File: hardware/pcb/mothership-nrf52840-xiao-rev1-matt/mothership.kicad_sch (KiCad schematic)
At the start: 46 parts, among them J1 HRO TYPE-C-31-M-12, J10 Screw_Terminal_ADB_SHIELD, J11 Screw_Terminal_ADB_VCC, J12 USB_FLEX_ADAPTER_SOLDER_PADS_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, J2 USB_FLEX_ADAPTER_SOLDER_PADS, J3 CONN_BATT, J4 CONN_MATRIX_BOT_L, J5 CONN_MATRIX_BOT_R, J6 CONN_MATRIX_TOP_L, J7 CONN_MATRIX_TOP_R, J8 SPI, J9 EC11, Q1 AO3401A, Q2 FDC6305N, SW1 SW_PWR, SW2 SW_EXT_RST, U1 NCP361SN, U2 XIAO_nRF52840, U3 MCP23017x-x-SS, U4 MCP23017x-x-SS, U5 DT1452-02SO, U6 HY2115-LB9D

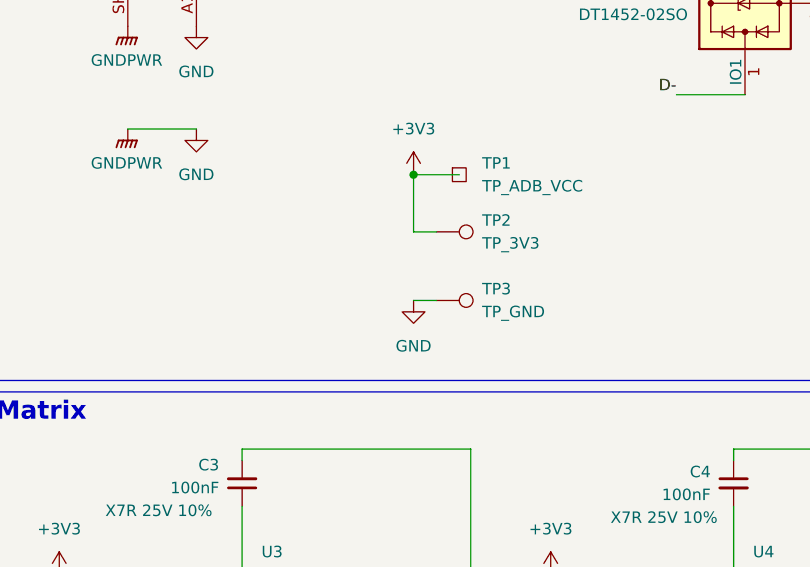
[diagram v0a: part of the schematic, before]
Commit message: sch: finalize the sch
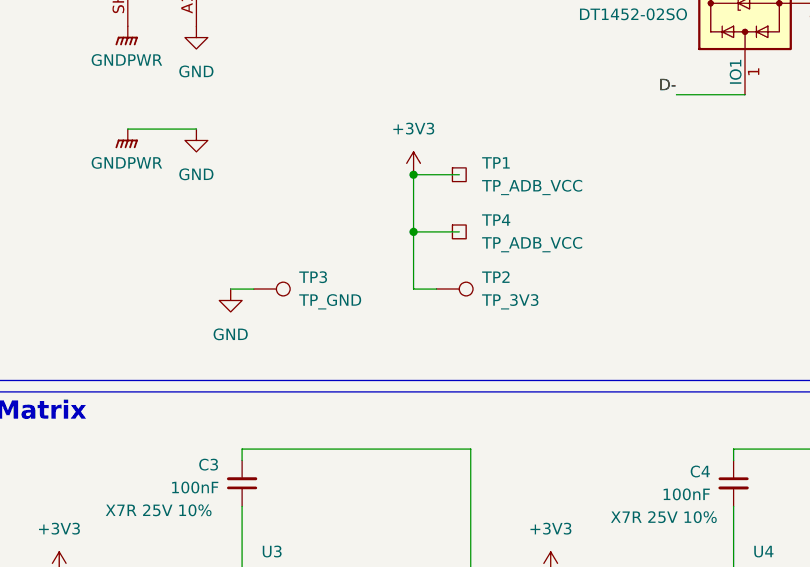
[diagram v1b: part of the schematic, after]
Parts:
- added TP4: TP_ADB_VCC, A9M0330:TestPoint_Pad_2.5x2.5mm, symbol A9M0330:TestPoint_Square
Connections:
- net +3V3: now also TP4.1
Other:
- moved on the sheet: TP3
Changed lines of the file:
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@@
 	)
 	(junction
+		(at 59.69 88.9)
+		(diameter 0)
+		(color 0 0 0 0)
+	)
+	(junction
 		(at 132.08 27.94)
 		(diameter 0)
@@
 	(wire
 		(pts
+			(xy 59.69 88.9) (xy 59.69 95.25)
+		)
+		(stroke
+			(width 0)
+			(type default)
+		)
+	)
+	(wire
+		(pts
 			(xy 140.97 60.96) (xy 140.97 62.23)
 		)
@@
 	(wire
 		(pts
+			(xy 59.69 95.25) (xy 62.23 95.25)
+		)
+		(stroke
+			(width 0)
+			(type default)
+		)
+	)
+	(wire
+		(pts
 			(xy 59.69 236.22) (xy 59.69 240.03)
 		)
@@
 	(wire
 		(pts
-			(xy 59.69 96.52) (xy 62.23 96.52)
+			(xy 39.37 95.25) (xy 41.91 95.25)
 		)
 		(stroke
@@
 	(wire
 		(pts
-			(xy 59.69 88.9) (xy 62.23 88.9)
+			(xy 59.69 88.9) (xy 64.77 88.9)
 		)
 		(stroke
@@
 	)
 	(symbol
+		(lib_id "A9M0330:TestPoint")
+		(at 62.23 95.25 270)
+		(unit 1)
+		(body_style 1)
+		(exclude_from_sim no)
+		(in_bom yes)
+		(on_board yes)
+		(in_pos_files yes)
+		(dnp no)
+		(fields_autoplaced yes)
+		(property "Reference" "TP2"
+			(at 67.31 93.9799 90)
+			(show_name no)
+			(do_not_autoplace no)
+			(effects
+				(font
+					(size 1.27 1.27)
+				)
+				(justify left)
+			)
+		)
+		(property "Value" "TP_3V3"
+			(at 67.31 96.5199 90)
+			(show_name no)
+			(do_not_autoplace no)
+			(effects
+				(font
+					(size 1.27 1.27)
+				)
+				(justify left)
+			)
+		)
+		(property "Footprint" "A9M0330:TestPoint_THTPad_D2.0mm_Drill1.0mm"
+			(at 62.23 100.33 0)
+			(hide yes)
+			(show_name no)
+			(do_not_autoplace no)
+			(effects
+				(font
+					(size 1.27 1.27)
+				)
+			)
+		)
+		(property "Datasheet" ""
+			(at 62.23 100.33 0)
+			(hide yes)
+			(show_name no)
+			(do_not_autoplace no)
+			(effects
+				(font
+					(size 1.27 1.27)
+				)
+			)
+		)
+		(property "Description" "test point"
+			(at 62.23 95.25 0)
+			(hide yes)
+			(show_name no)
+			(do_not_autoplace no)
+			(effects
+				(font
+					(size 1.27 1.27)
+				)
+			)
+		)
+		(pin "1"
+		)
+		(instances
+			(project "mothership"
+				(path "/02dc08fe-8ec4-4078-b85a-ecd1690e4fdc"
+					(reference "TP2")
+					(unit 1)
+				)
+			)
+		)
+	)
+	(symbol
 		(lib_id "power:+3V3")
 		(at 74.93 127 0)
@@
 	)
 	(symbol
-		(lib_id "A9M0330:TestPoint")
-		(at 62.23 88.9 270)
-		(unit 1)
-		(body_style 1)
-		(exclude_from_sim no)
-		(in_bom yes)
-		(on_board yes)
-		(in_pos_files yes)
-		(dnp no)
-		(fields_autoplaced yes)
-		(property "Reference" "TP2"
-			(at 67.31 87.6299 90)
-			(show_name no)
-			(do_not_autoplace no)
-			(effects
-				(font
-					(size 1.27 1.27)
-				)
-				(justify left)
-			)
-		)
-		(property "Value" "TP_3V3"
-			(at 67.31 90.1699 90)
-			(show_name no)
-			(do_not_autoplace no)
-			(effects
-				(font
-					(size 1.27 1.27)
-				)
-				(justify left)
-			)
-		)
-		(property "Footprint" "A9M0330:TestPoint_THTPad_D2.0mm_Drill1.0mm"
-			(at 62.23 93.98 0)
-			(hide yes)
-			(show_name no)
-			(do_not_autoplace no)
-			(effects
-				(font
-					(size 1.27 1.27)
-				)
-			)
-		)
-		(property "Datasheet" ""
-			(at 62.23 93.98 0)
-			(hide yes)
-			(show_name no)
-			(do_not_autoplace no)
-			(effects
-				(font
-					(size 1.27 1.27)
-				)
-			)
-		)
-		(property "Description" "test point"
-			(at 62.23 88.9 0)
-			(hide yes)
-			(show_name no)
-			(do_not_autoplace no)
-			(effects
-				(font
-					(size 1.27 1.27)
-				)
-			)
-		)
-		(pin "1"
-		)
-		(instances
-			(project "mothership"
-				(path "/02dc08fe-8ec4-4078-b85a-ecd1690e4fdc"
-					(reference "TP2")
-					(unit 1)
-				)
-			)
-		)
-	)
-	(symbol
 		(lib_id "power:GND")
 		(at 337.82 147.32 0)
@@
 	(symbol
 		(lib_id "power:GND")
-		(at 59.69 96.52 0)
+		(at 39.37 95.25 0)
 		(unit 1)
 		(body_style 1)
@@
 		(fields_autoplaced yes)
 		(property "Reference" "#PWR011"
-			(at 59.69 102.87 0)
+			(at 39.37 101.6 0)
 			(hide yes)
 			(show_name no)
@@
 		)
 		(property "Value" "GND"
-			(at 59.69 101.6 0)
+			(at 39.37 100.33 0)
 			(show_name no)
 			(do_not_autoplace no)
@@
 		)
 		(property "Footprint" ""
-			(at 59.69 96.52 0)
+			(at 39.37 95.25 0)
 			(hide yes)
 			(show_name no)
@@
 		)
 		(property "Datasheet" ""
-			(at 59.69 96.52 0)
+			(at 39.37 95.25 0)
 			(hide yes)
 			(show_name no)
@@
 		)
 		(property "Description" "Power symbol creates a global label with name \"GND\" , ground"
-			(at 59.69 96.52 0)
+			(at 39.37 95.25 0)
 			(hide yes)
 			(show_name no)
@@
 	(symbol
 		(lib_id "A9M0330:TestPoint")
-		(at 62.23 96.52 270)
+		(at 41.91 95.25 270)
 		(unit 1)
 		(body_style 1)
@@
 		(fields_autoplaced yes)
 		(property "Reference" "TP3"
-			(at 67.31 95.2499 90)
+			(at 46.99 93.9799 90)
 			(show_name no)
 			(do_not_autoplace no)
@@
 		)
 		(property "Value" "TP_GND"
-			(at 67.31 97.7899 90)
+			(at 46.99 96.5199 90)
 			(show_name no)
 			(do_not_autoplace no)
@@
 		)
 		(property "Footprint" "A9M0330:TestPoint_THTPad_2.0x2.0mm_Drill1.0mm"
-			(at 62.23 101.6 0)
+			(at 41.91 100.33 0)
 			(hide yes)
 			(show_name no)
@@
 		)
 		(property "Datasheet" ""
-			(at 62.23 101.6 0)
+			(at 41.91 100.33 0)
 			(hide yes)
 			(show_name no)
@@
 		)
 		(property "Description" "test point"
-			(at 62.23 96.52 0)
+			(at 41.91 95.25 0)
 			(hide yes)
 			(show_name no)
@@
 					(unit 1)
 				)
+			)
+		)
+	)
+	(symbol
+		(lib_id "A9M0330:TestPoint_Square")
+		(at 64.77 88.9 0)
+		(unit 1)
+		(body_style 1)
+		(exclude_from_sim no)
+		(in_bom yes)
+		(on_board yes)
+		(in_pos_files yes)
+		(dnp no)
+		(property "Reference" "TP4"
+			(at 67.31 87.6299 0)
+			(show_name no)
+			(do_not_autoplace no)
+			(effects
+				(font
+					(size 1.27 1.27)
+				)
+				(justify left)
+			)
+		)
+		(property "Value" "TP_ADB_VCC"
+			(at 67.31 90.17 0)
+			(show_name no)
+			(do_not_autoplace no)
+			(effects
+				(font
+					(size 1.27 1.27)
+				)
+				(justify left)
+			)
+		)
+		(property "Footprint" "A9M0330:TestPoint_Pad_2.5x2.5mm"
+			(at 69.85 88.9 0)
+			(hide yes)
+			(show_name no)
+			(do_not_autoplace no)
+			(effects
+				(font
+					(size 1.27 1.27)
+				)
+			)
+		)
+		(property "Datasheet" "~"
+			(at 69.85 88.9 0)
+			(hide yes)
+			(show_name no)
+			(do_not_autoplace no)
+			(effects
+				(font
+					(size 1.27 1.27)
+				)
+			)
+		)
+		(property "Description" "test point"
+			(at 64.77 88.9 0)
+			(hide yes)
+			(show_name no)
+			(do_not_autoplace no)
+			(effects
+				(font
+					(size 1.27 1.27)
+				)
+			)
+		)
+		(pin "1"
+		)
+		(instances
+			(project "mothership"
+				(path "/02dc08fe-8ec4-4078-b85a-ecd1690e4fdc"
+					(reference "TP4")
+					(unit 1)
+				)
